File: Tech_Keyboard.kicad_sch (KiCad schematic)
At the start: 19 parts, among them U1 Arduino_Pro_Micro

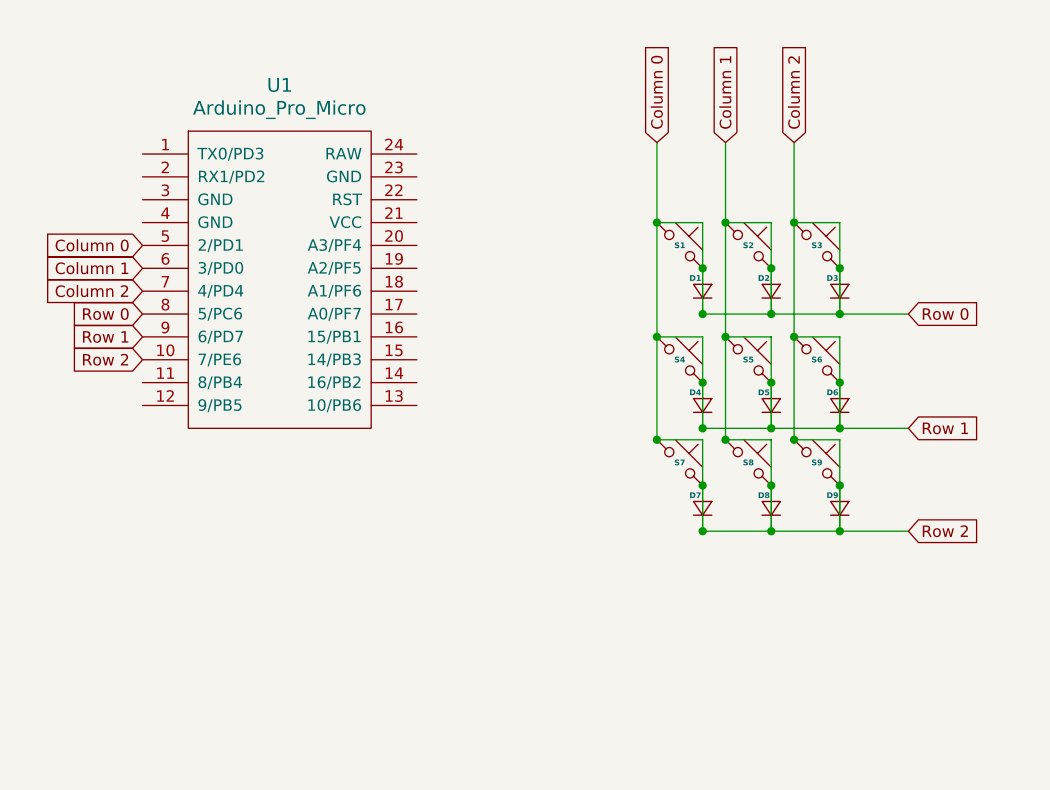
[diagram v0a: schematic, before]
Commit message: Update Tech_Keyboard.kicad_sch
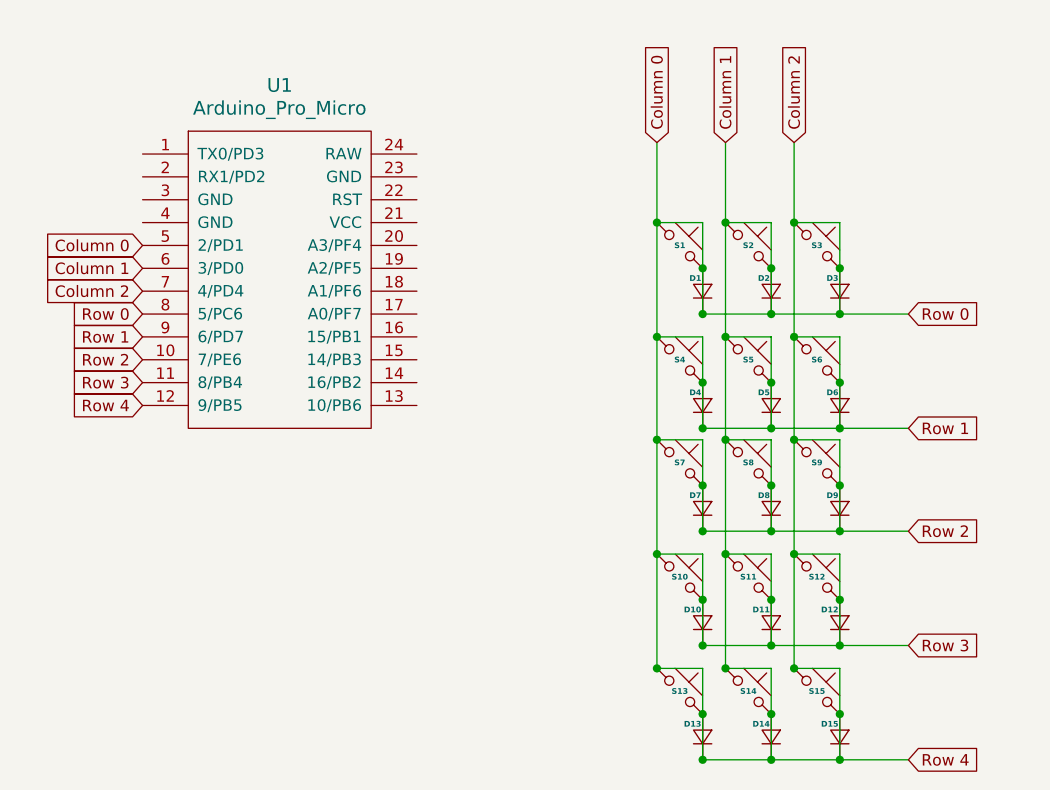
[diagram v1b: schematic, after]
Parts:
- added D10, D11, D12, D13, D14, D15: ~, symbol ScottoKeebs:Placeholder_Diode
- added S10, S11, S12, S13, S14, S15: ~, symbol ScottoKeebs:Placeholder_Keyswitch
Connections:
- net Column 0: now also U1.11 (8/PB4), U1.12 (9/PB5), D10.1 (K), D10.2 (A), D11.1 (K), D11.2 (A), D12.1 (K), D12.2 (A), D13.1 (K), D13.2 (A), D14.1 (K), D14.2 (A), D15.1 (K), D15.2 (A), S10.1, S10.2, S11.1, S11.2, S12.1, S12.2, S13.1, S13.2, S14.1, S14.2, S15.1, S15.2

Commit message: Update Tech_Keyboard.kicad_sch
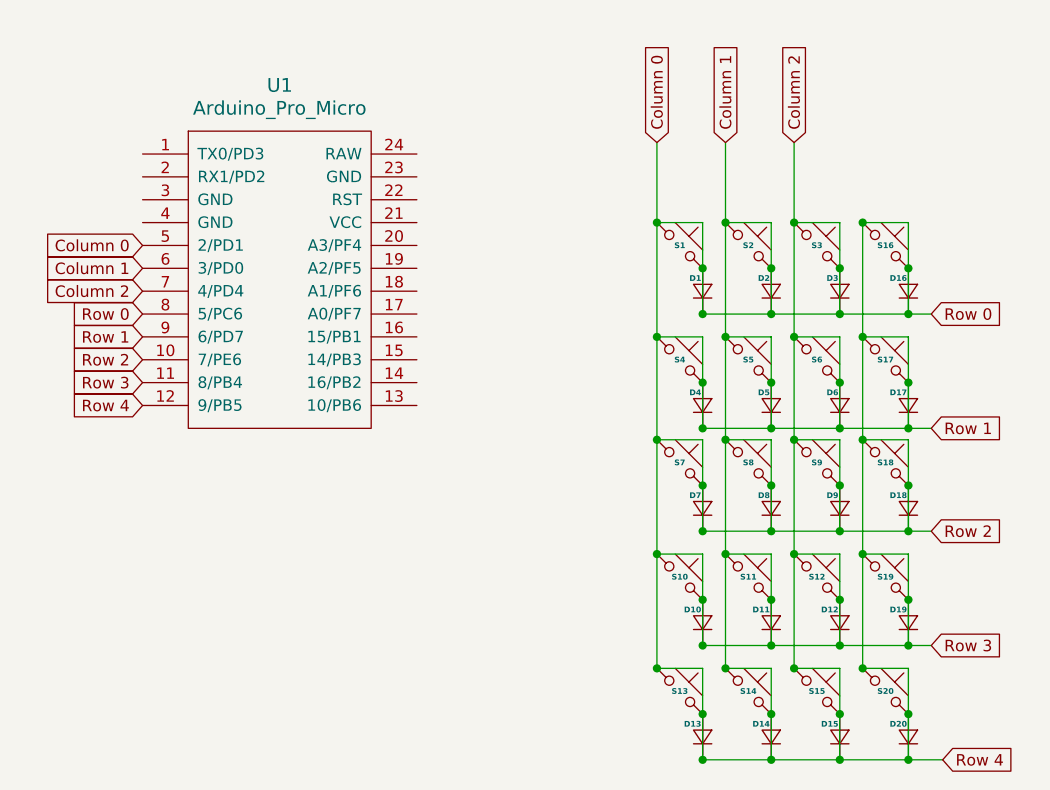
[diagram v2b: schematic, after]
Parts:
- added D16, D17, D18, D19, D20: ~, symbol ScottoKeebs:Placeholder_Diode
- added S16, S17, S18, S19, S20: ~, symbol ScottoKeebs:Placeholder_Keyswitch
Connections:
- net Column 0: now also D16.1 (K), D16.2 (A), D17.1 (K), D17.2 (A), D18.1 (K), D18.2 (A), D19.1 (K), D19.2 (A), D20.1 (K), D20.2 (A), S16.1, S16.2, S17.1, S17.2, S18.1, S18.2, S19.1, S19.2, S20.1, S20.2
